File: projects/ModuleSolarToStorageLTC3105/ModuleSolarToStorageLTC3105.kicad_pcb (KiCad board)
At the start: 2 copper layers, 15 x 13 mm, 10 parts, among them U1 LTC3105EMS-PBF

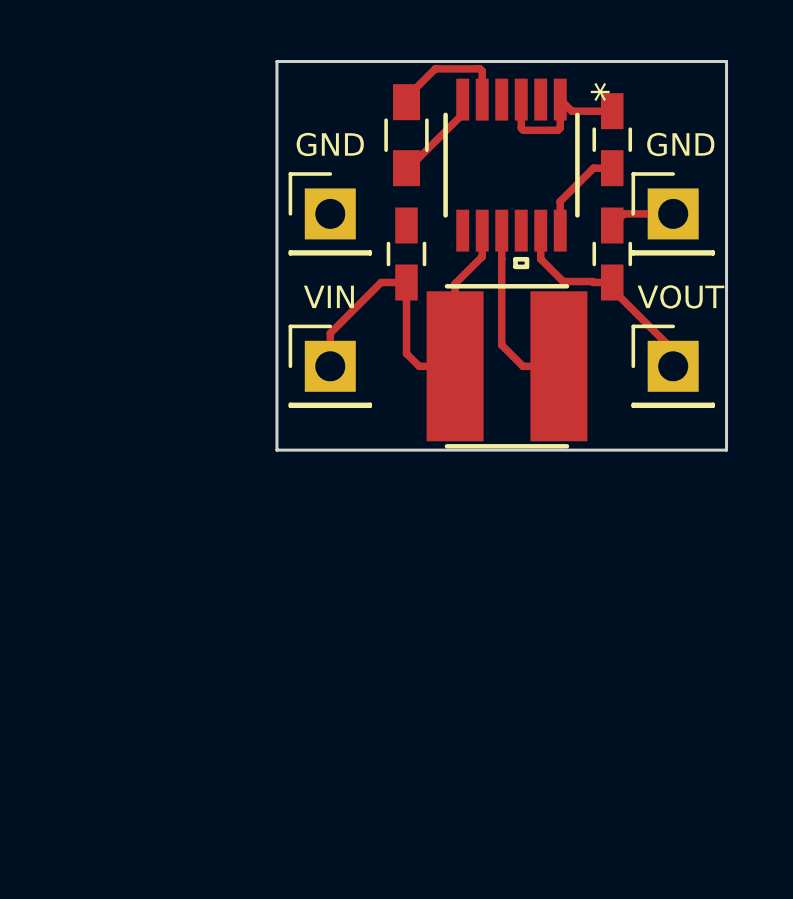
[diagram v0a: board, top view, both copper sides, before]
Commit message: KiCad ModuleSolarToStorageLTC3105 Rev2
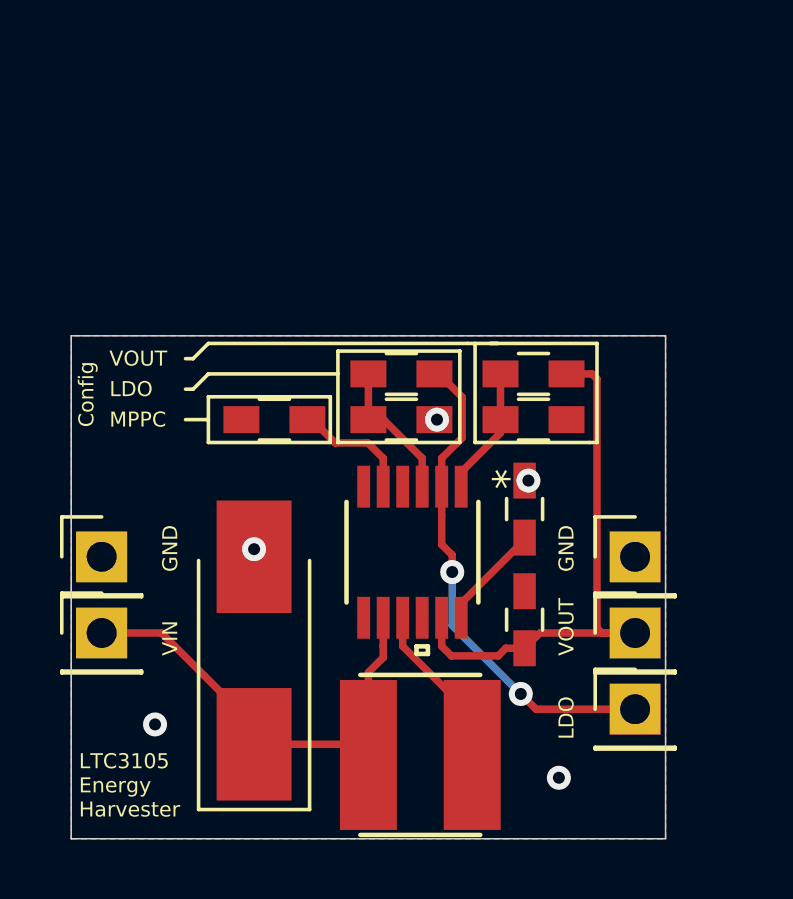
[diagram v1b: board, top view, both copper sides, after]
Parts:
- removed C4: C_Small, Capacitors_SMD:C_0603_HandSoldering
- removed GND_EXTERNAL1, GND_EXTERNAL2, VIN_EXTERNAL2, VOUT_EXTERNAL1: Conn_01x01_Female, Socket_Strips:Socket_Strip_Straight_1x01_Pitch2.54mm
- added C1: ??uF, Capacitors_SMD:C_0603_HandSoldering, F.Cu at (134.7, 83.4)
- added J1: VIN, Socket_Strips:Socket_Strip_Straight_1x01_Pitch2.54mm, F.Cu at (120.7, 83.8)
- added J2: GND, Socket_Strips:Socket_Strip_Straight_1x01_Pitch2.54mm, F.Cu at (120.7, 81.3)
- added J3: VOUT, Socket_Strips:Socket_Strip_Straight_1x01_Pitch2.54mm, F.Cu at (138.4, 83.8)
- added J4: LDO, Socket_Strips:Socket_Strip_Straight_1x01_Pitch2.54mm, F.Cu at (138.4, 86.4)
- added J5: GND, Socket_Strips:Socket_Strip_Straight_1x01_Pitch2.54mm, F.Cu at (138.4, 81.3)
- added R1: R_Small, Resistors_SMD:R_0603_HandSoldering, F.Cu at (135.0, 75.2)
- added R2: R_Small, Resistors_SMD:R_0603_HandSoldering, F.Cu at (135.0, 76.7)
- added R4: R_Small, Resistors_SMD:R_0603_HandSoldering, F.Cu at (130.6, 76.7)
- added R5: R_Small, Resistors_SMD:R_0603_HandSoldering, F.Cu at (126.4, 76.7)
- C2: value C_Small -> 1uF
- C3: value C_Small -> ??uF; footprint Capacitors_SMD:C_0603_HandSoldering -> Capacitors_Tantalum_SMD:CP_Tantalum_Case-U_EIA-6032-15_Hand
- L1: value L_Small -> 10uH
- moved C3 17.8 mm to (125.7, 84.4)
- moved U1 13.3 mm to (131.0, 81.1)
- moved L1 13.3 mm to (131.3, 87.9), turned to 180 degrees
- moved C2 9.37 mm to (134.7, 79.7)
- moved R3 7.96 mm to (130.6, 75.2), turned to 180 degrees
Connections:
- C2 pad 1: VIN -> Net-(C2-Pad1)
- C2 pad 2: FBLDO_PROGRAMMING -> GND
- C3 pad 1: VOUT -> VIN
- C3 pad 2: FBLDO_PROGRAMMING -> GND
- L1 pad 1: VIN -> Net-(L1-Pad1)
- L1 pad 2: SW -> VIN
- R3 pad 1: MPPC_PROGRAMMING -> LDO
- R3 pad 2: FBLDO_PROGRAMMING -> Net-(R3-Pad2)
- U1 pad 1: FBLDO_PROGRAMMING -> Net-(R1-Pad2)
- U1 pad 12: AUX -> Net-(C2-Pad1)
- U1 pad 2: (no net) -> LDO
- U1 pad 3: FBLDO_PROGRAMMING -> Net-(R3-Pad2)
- U1 pad 5: MPPC_PROGRAMMING -> Net-(R5-Pad1)
- U1 pad 6: FBLDO_PROGRAMMING -> GND
- U1 pad 7: FBLDO_PROGRAMMING -> GND
- U1 pad 9: SW -> Net-(L1-Pad1)
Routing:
- net LDO: track 0.00 -> 16.5 mm, vias 0 -> 2
- net VOUT: track 7.29 -> 18.6 mm
- net FBLDO_PROGRAMMING: track 10.4 -> 0.00 mm
- net SW: track 6.01 -> 0.00 mm
- net Net-(L1-Pad1): track 0.00 -> 5.53 mm
- net Net-(R3-Pad2): track 0.00 -> 4.80 mm
- net Net-(R1-Pad2): track 0.00 -> 4.30 mm
- net MPPC_PROGRAMMING: track 4.05 -> 0.00 mm
- net Net-(R5-Pad1): track 0.00 -> 4.01 mm
- net Net-(C2-Pad1): track 0.00 -> 3.55 mm
- net AUX: track 3.17 -> 0.00 mm
- net VIN: track 13.4 -> 15.7 mm
- net GND: vias 0 -> 5
- added copper zone on B.Cu, net GND
- added copper zone on F.Cu, net GND
- removed copper zone on B.Cu, net FBLDO_PROGRAMMING
- removed copper zone on F.Cu, net FBLDO_PROGRAMMING
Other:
- board size 15 x 13 mm -> 19.8 x 16.8 mm
- rule pad_to_mask_clearance: 0 -> 0.051
- board text added: "Config"
- board text added: "LDO"
- board text added: "LTC3105 Energy Harvester"
- board text added: "MPPC"
- board text added: "ModuleSolarToStorageLTC3105 2019-03-29 Rev2"
- board text removed: "SolarToStorage LTC3105 2019-02-18 Rev 1"
